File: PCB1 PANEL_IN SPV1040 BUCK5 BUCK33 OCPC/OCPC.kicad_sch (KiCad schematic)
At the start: 10 parts, among them J7 Conn_01x02_Pin, J8 Conn_01x01_Pin, J9 Conn_01x02_Pin, U14 TPS2557DRBR

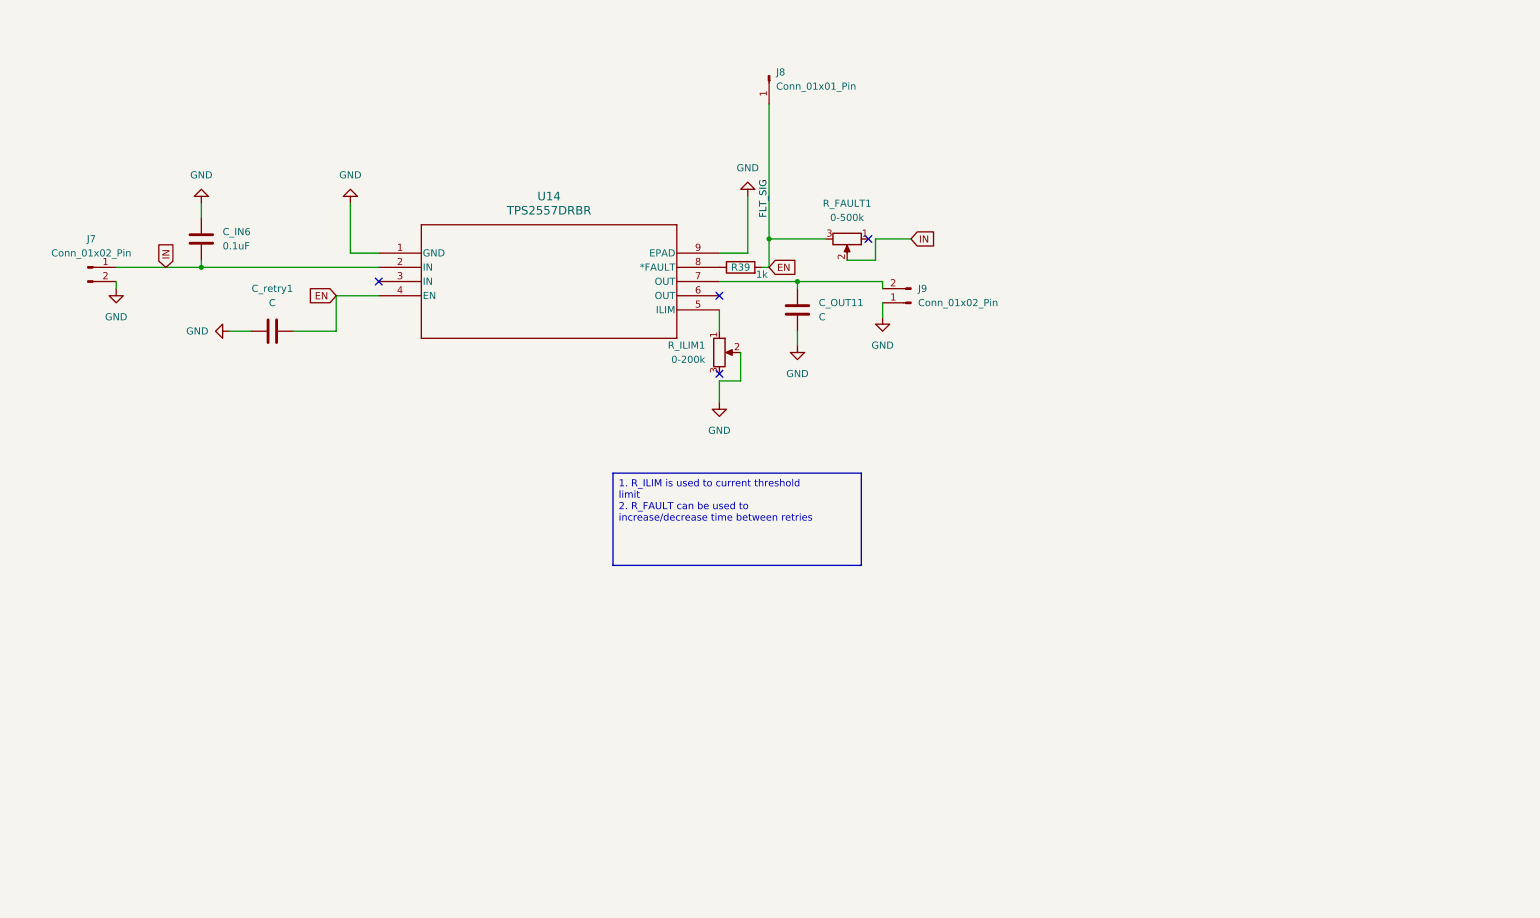
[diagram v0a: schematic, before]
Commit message: EDITS NTH
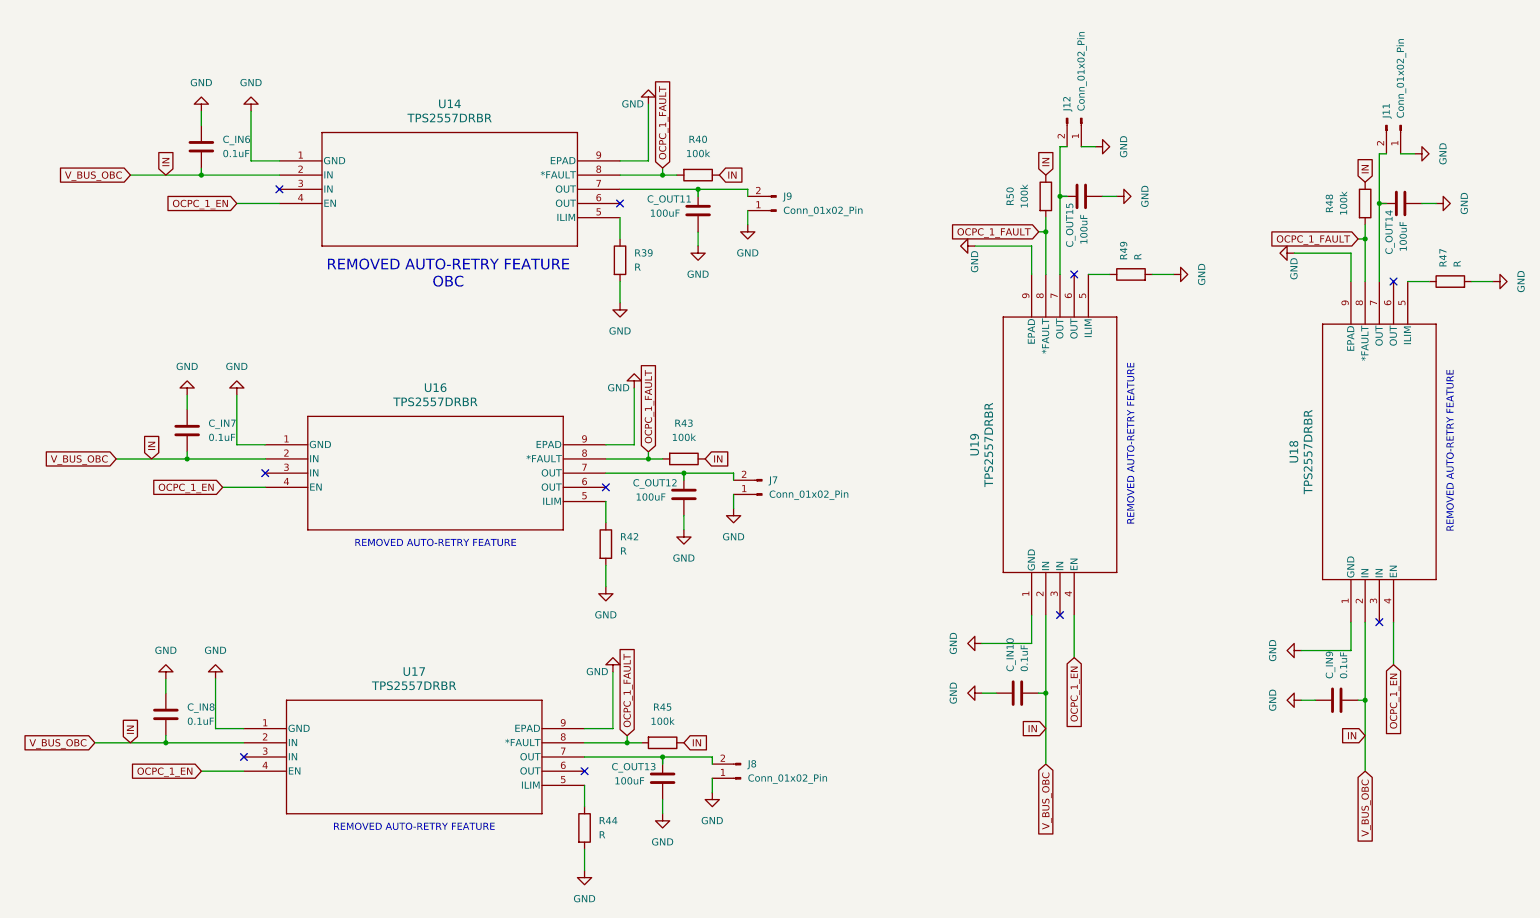
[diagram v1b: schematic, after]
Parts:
- removed C_retry1: C, Capacitor_SMD:C_0504_1310Metric, symbol Device:C
- removed J8: Conn_01x01_Pin, Connector_PinHeader_2.54mm:PinHeader_1x01_P2.54mm_Vertical, symbol Connector:Conn_01x01_Pin
- removed R_FAULT1: 0-500k, symbol Device:R_Potentiometer
- removed R_ILIM1: 0-200k, symbol Device:R_Potentiometer
- added C_IN10, C_IN7, C_IN8, C_IN9: 0.1uF, Capacitor_SMD:C_0603_1608Metric, symbol Device:C
- added C_OUT12, C_OUT13, C_OUT14, C_OUT15: 100uF, Capacitor_SMD:C_0504_1310Metric, symbol Device:C
- added J11, J12, J8: Conn_01x02_Pin, Connector_PinHeader_2.54mm:PinHeader_1x02_P2.54mm_Vertical, symbol Connector:Conn_01x02_Pin
- added R40, R43, R45, R48, R50: 100k, Resistor_SMD:R_01005_0402Metric_Pad0.57x0.30mm_HandSolder, symbol Device:R
- added R42, R44, R47, R49: R, Resistor_SMD:R_0603_1608Metric_Pad0.98x0.95mm_HandSolder, symbol Device:R
- added U16, U17, U18, U19: TPS2557DRBR, TPS2557:DRB8_2P4X1P65, symbol TPS2557:TPS2557DRBR
- C_OUT11: value C -> 100uF
- R39: value 1k -> R; footprint Resistor_SMD:R_1812_4532Metric -> Resistor_SMD:R_0603_1608Metric_Pad0.98x0.95mm_HandSolder
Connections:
- net GND: now also J7.1 (Pin_1), R39.2, C_IN10.1, C_IN7.1, C_IN8.1, C_IN9.1, C_OUT12.1, C_OUT13.1, C_OUT14.1, C_OUT15.1, J11.1 (Pin_1), J12.1 (Pin_1), J8.1 (Pin_1), R42.2, R44.2, R47.2, R49.2, U16.1 (GND), U16.9 (EPAD), U17.1 (GND), U17.9 (EPAD), U18.1 (GND), U18.9 (EPAD), U19.1 (GND), U19.9 (EPAD); no longer J7.2 (Pin_2)
- net IN: now also C_IN10.2, C_IN7.2, C_IN8.2, C_IN9.2, R40.1, R43.1, R45.1, R48.1, R50.1, U16.2 (IN), U17.2 (IN), U18.2 (IN), U19.2 (IN); no longer J7.1 (Pin_1)
- net at U14.5 (ILIM): now also R39.1
- net OCPC_1_FAULT: now reaches U14.8 (*FAULT)
- net OCPC_1_FAULT: now also R40.2, R43.2, R45.2, R48.2, R50.2, U16.8 (*FAULT), U17.8 (*FAULT), U18.8 (*FAULT), U19.8 (*FAULT); no longer R39.1
- net EN renamed OCPC_1_EN
- net OCPC_1_EN: now also U16.4 (EN), U17.4 (EN), U18.4 (EN), U19.4 (EN); no longer R39.2
- new net: R47.1, U18.5 (ILIM)
- new net: R44.1, U17.5 (ILIM)
- new net: C_OUT13.2, J8.2 (Pin_2), U17.7 (OUT)
- new net: R49.1, U19.5 (ILIM)
- new net: C_OUT14.2, J11.2 (Pin_2), U18.7 (OUT)
- new net: C_OUT15.2, J12.2 (Pin_2), U19.7 (OUT)
- new net: R42.1, U16.5 (ILIM)
- new net: C_OUT12.2, J7.2 (Pin_2), U16.7 (OUT)
- no-connect marks 4 -> 10
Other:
- note added: "REMOVED AUTO-RETRY FEATURE"
- note added: "REMOVED AUTO-RETRY FEATURE OBC"
- moved on the sheet: C_IN6, C_OUT11, J9, U14
